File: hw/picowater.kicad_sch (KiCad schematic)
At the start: 22 parts, among them J1 GPIO Pins, J2 Power In, J3 +5V Pins, J4 UART, J5 Power Out, J6 RTC, J7 GPIO2, U1 Pico

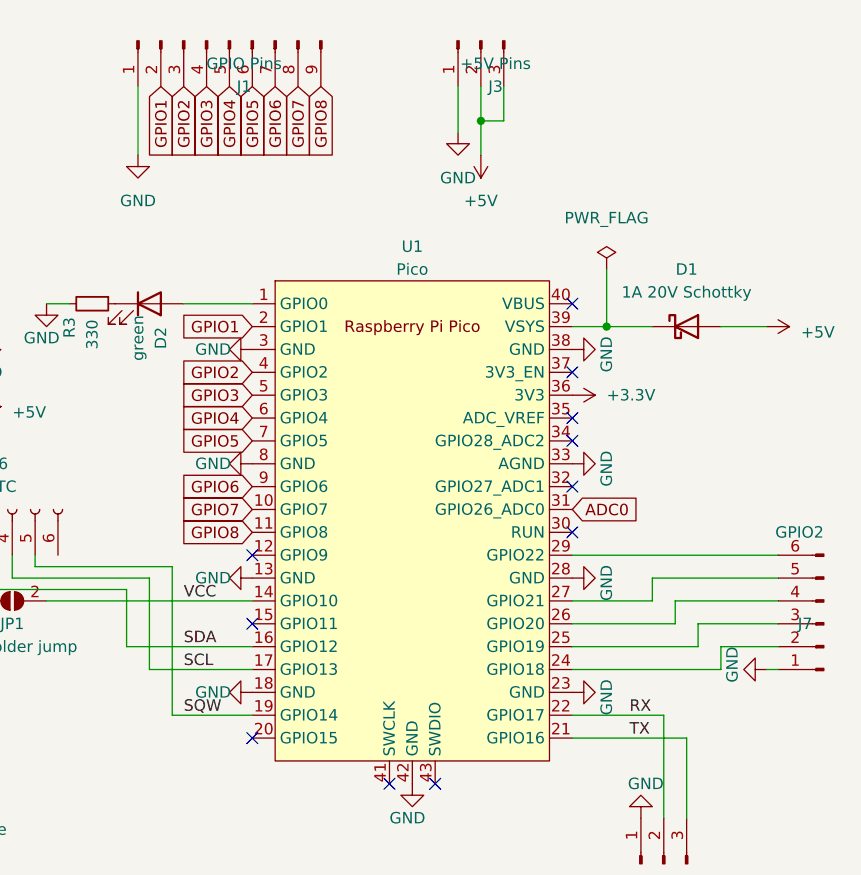
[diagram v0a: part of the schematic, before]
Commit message: [hw] update pcb
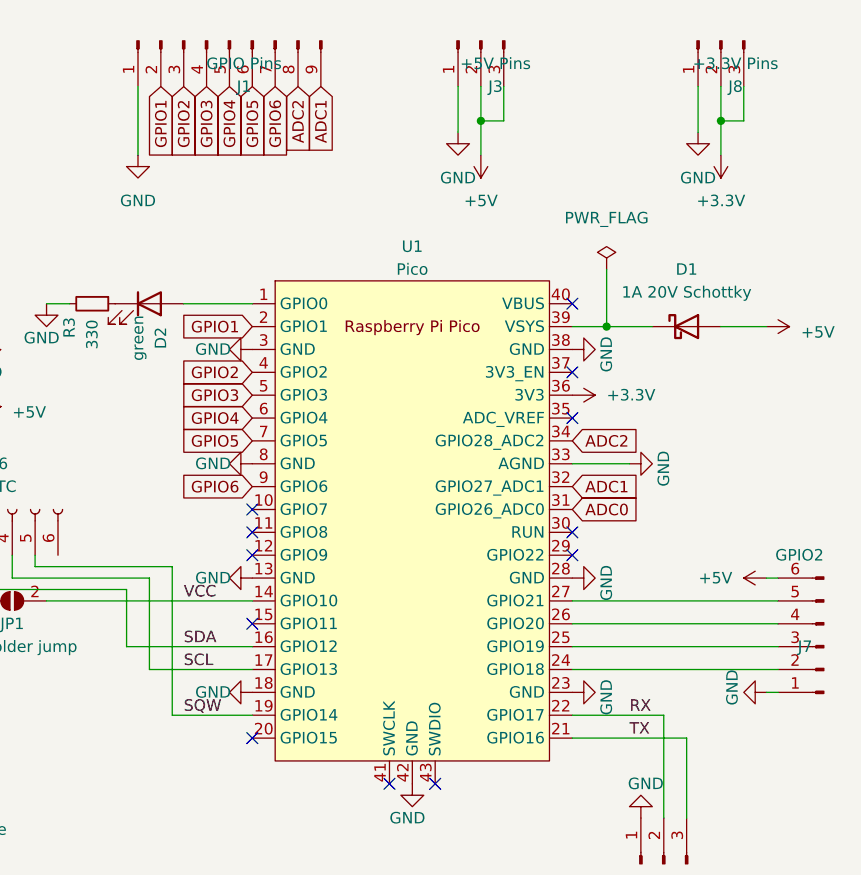
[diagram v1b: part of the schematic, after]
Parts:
- added J8: +3.3V Pins, Connector_PinHeader_2.54mm:PinHeader_1x03_P2.54mm_Vertical, symbol Connector:Conn_01x03_Pin
- R1, R2: footprint Resistor_THT:R_Axial_DIN0204_L3.6mm_D1.6mm_P5.08mm_Horizontal -> Resistor_THT:R_Axial_DIN0204_L3.6mm_D1.6mm_P7.62mm_Horizontal
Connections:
- net +3.3V: now also J8.2 (Pin_2), J8.3 (Pin_3)
- net +5V: now also J7.6 (Pin_6)
- net GND: now also J8.1 (Pin_1)
- net at U1.29 (GPIO22): no longer J7.6 (Pin_6)
- net ADC1: now reaches U1.32 (GPIO27_ADC1)
- net ADC1: now also J1.9 (Pin_9)
- net ADC2: now reaches U1.34 (GPIO28_ADC2)
- net ADC2: now also J1.8 (Pin_8)
- net GPIO7: no longer names the net of U1.10 (GPIO7)
- net GPIO7: no longer J1.8 (Pin_8)
- net GPIO8: no longer names the net of U1.11 (GPIO8)
- net GPIO8: no longer J1.9 (Pin_9)
- no-connect marks 11 -> 12
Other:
- moved on the sheet: J7

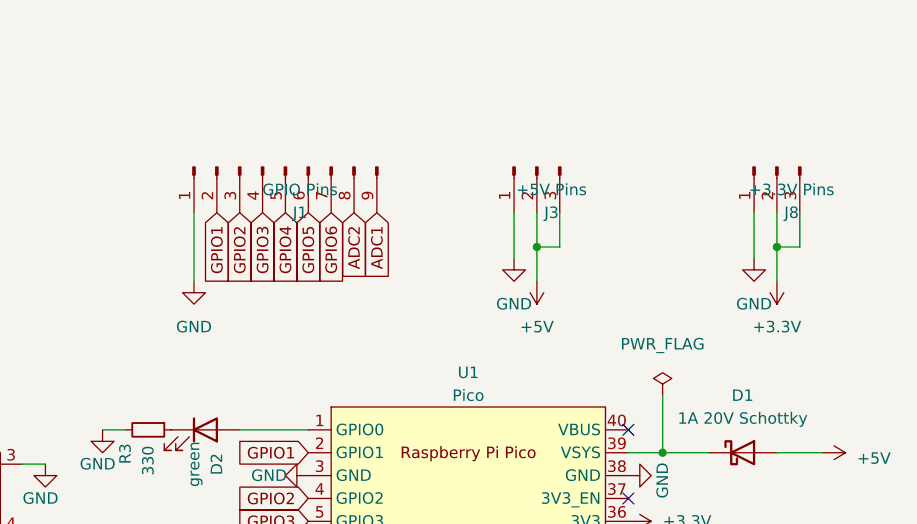
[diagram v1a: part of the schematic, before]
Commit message: [hw] v0.3 release
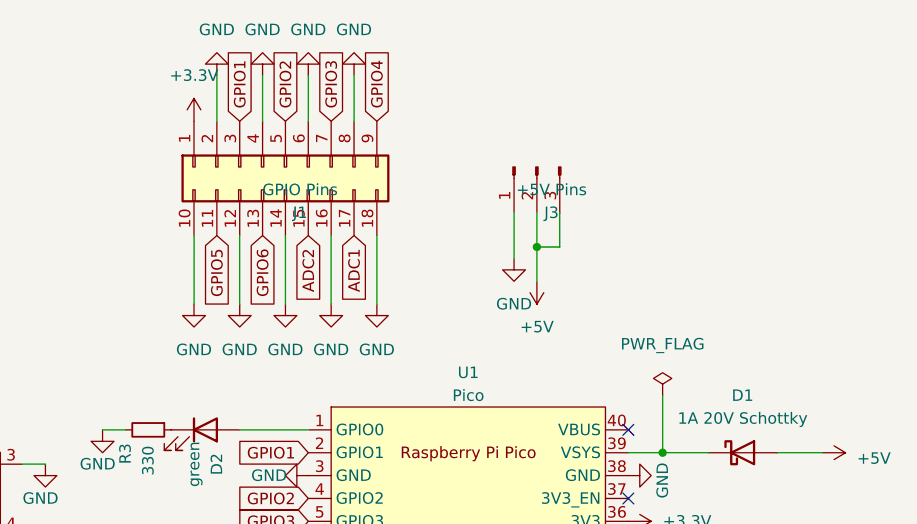
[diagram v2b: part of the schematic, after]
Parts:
- removed J8: +3.3V Pins, Connector_PinHeader_2.54mm:PinHeader_1x03_P2.54mm_Vertical, symbol Connector:Conn_01x03_Pin
- J1: footprint Connector_PinHeader_2.54mm:PinHeader_1x09_P2.54mm_Vertical -> Connector_PinHeader_2.54mm:PinHeader_2x09_P2.54mm_Vertical; symbol Connector:Conn_01x09_Pin -> Connector_Generic:Conn_02x09_Top_Bottom
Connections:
- net +3.3V: now also J1.1 (Pin_1)
- net ADC1: now also J1.17 (Pin_17); no longer J1.9 (Pin_9)
- net ADC2: now also J1.15 (Pin_15); no longer J1.8 (Pin_8)
- net GND: now also J1.10 (Pin_10), J1.12 (Pin_12), J1.14 (Pin_14), J1.16 (Pin_16), J1.18 (Pin_18), J1.2 (Pin_2), J1.4 (Pin_4), J1.6 (Pin_6), J1.8 (Pin_8); no longer J1.1 (Pin_1)
- net GPIO1: now also J1.3 (Pin_3); no longer J1.2 (Pin_2)
- net GPIO2: now also J1.5 (Pin_5); no longer J1.3 (Pin_3)
- net GPIO3: now also J1.7 (Pin_7); no longer J1.4 (Pin_4)
- net GPIO4: now also J1.9 (Pin_9); no longer J1.5 (Pin_5)
- net GPIO5: now also J1.11 (Pin_11); no longer J1.6 (Pin_6)
- net GPIO6: now also J1.13 (Pin_13); no longer J1.7 (Pin_7)
